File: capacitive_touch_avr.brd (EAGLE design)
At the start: 24.1 x 46 mm, 10 parts, among them J2 JACK-2.1MM

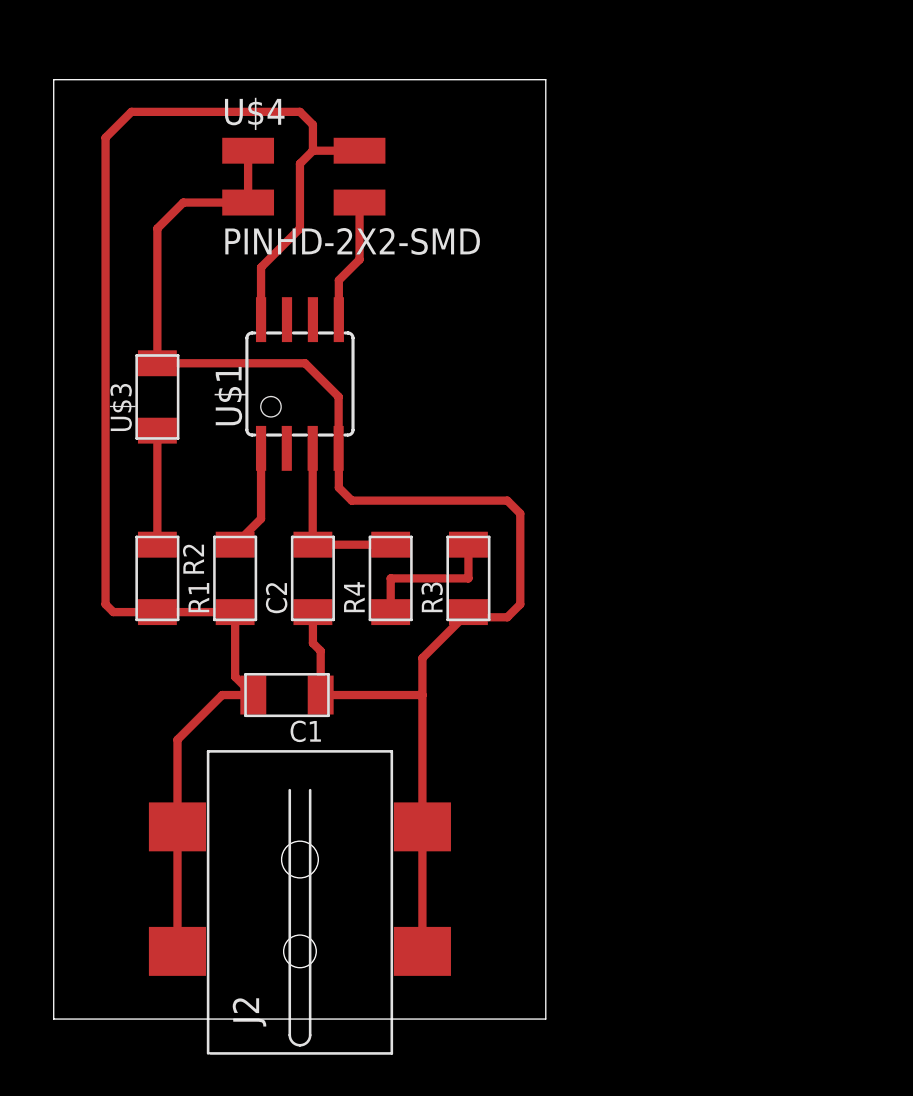
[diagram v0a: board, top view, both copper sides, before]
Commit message: Version 1. Touch pad + full wiring
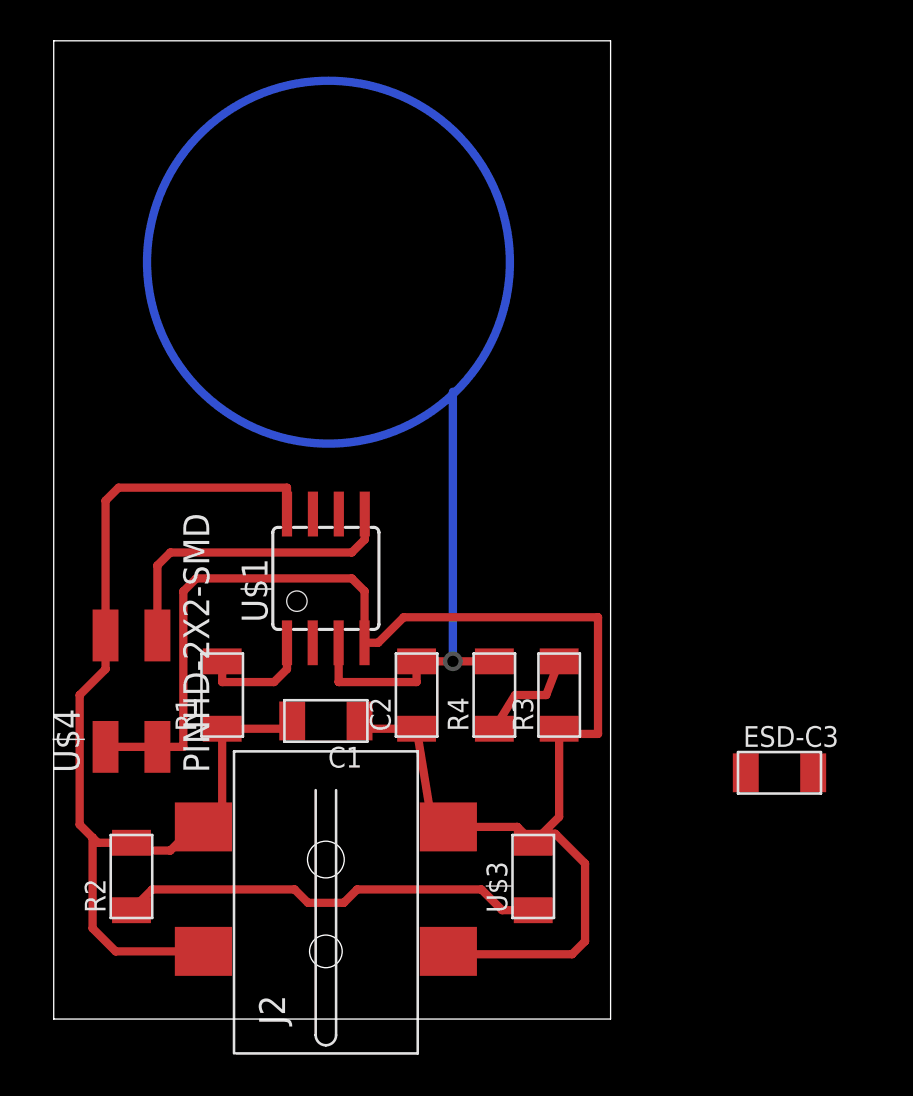
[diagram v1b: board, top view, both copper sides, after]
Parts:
- added ESD-C3: 0.1uF, fab:C1206FAB
- moved U$3 29.9 mm to (23.5, 6.99)
- moved U$4 26.7 mm to (3.81, 15.9), turned to 90 degrees
- moved R2 14.7 mm to (3.81, 6.99), turned to 90 degrees
- moved U$1 9.61 mm to (13.3, 21.6)
- moved C2 7.65 mm to (17.8, 15.9)
- moved R4 7.65 mm to (21.6, 15.9)
- moved R3 7.24 mm to (24.8, 15.9)
- moved R1 5.75 mm to (8.26, 15.9)
- moved C1 2.29 mm to (13.3, 14.6)
- moved J2 1.27 mm to (13.3, 5.71)
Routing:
- net VCC: track 72.6 -> 53.0 mm
- net N$3: track 5.59 -> 21.1 mm
- net CPIN: track 8.53 -> 23.8 mm, vias 0 -> 1
- net MOSI: track 6.16 -> 15.4 mm
- net GND: track 71.7 -> 76.1 mm
- net N$4: track 7.11 -> 5.23 mm
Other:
- board size 24.1 x 46 mm -> 27.3 x 47.9 mm
